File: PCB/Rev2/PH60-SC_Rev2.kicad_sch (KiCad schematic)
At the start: 43 parts, among them J1 Conn_01x02_Pin, J3 USB_C_Receptacle_USB2.0_14P, J4 Conn_01x02_Pin, U1 nRF52840, X2 32.768kHz, X3 Crystal_Generic

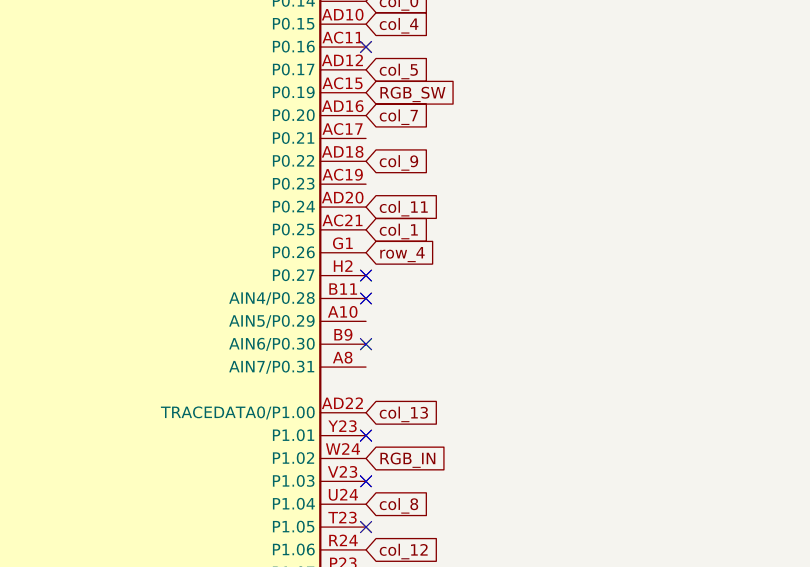
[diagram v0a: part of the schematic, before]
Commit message: layout and drc
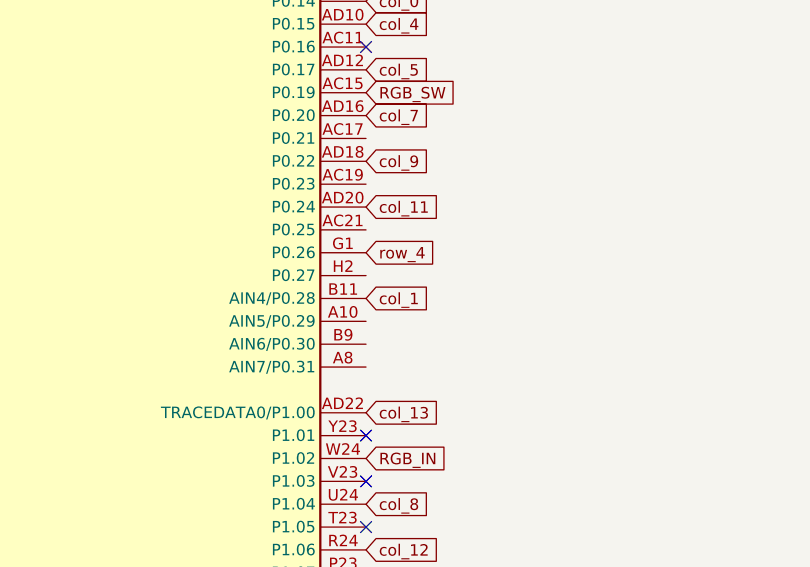
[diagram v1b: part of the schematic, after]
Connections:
- net col_1: now also U1.B11 (AIN4/P0.28); no longer U1.AC21 (P0.25)
- no-connect marks 18 -> 15
